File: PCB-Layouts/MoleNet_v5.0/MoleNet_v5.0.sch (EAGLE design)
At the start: 29 parts, among them Q1 MOSFET-NCHANNELBSS138, U1 STM32L073RZT6, U2 SN74LVC1G240DBVR, X1 734120110, Y1 16MHz

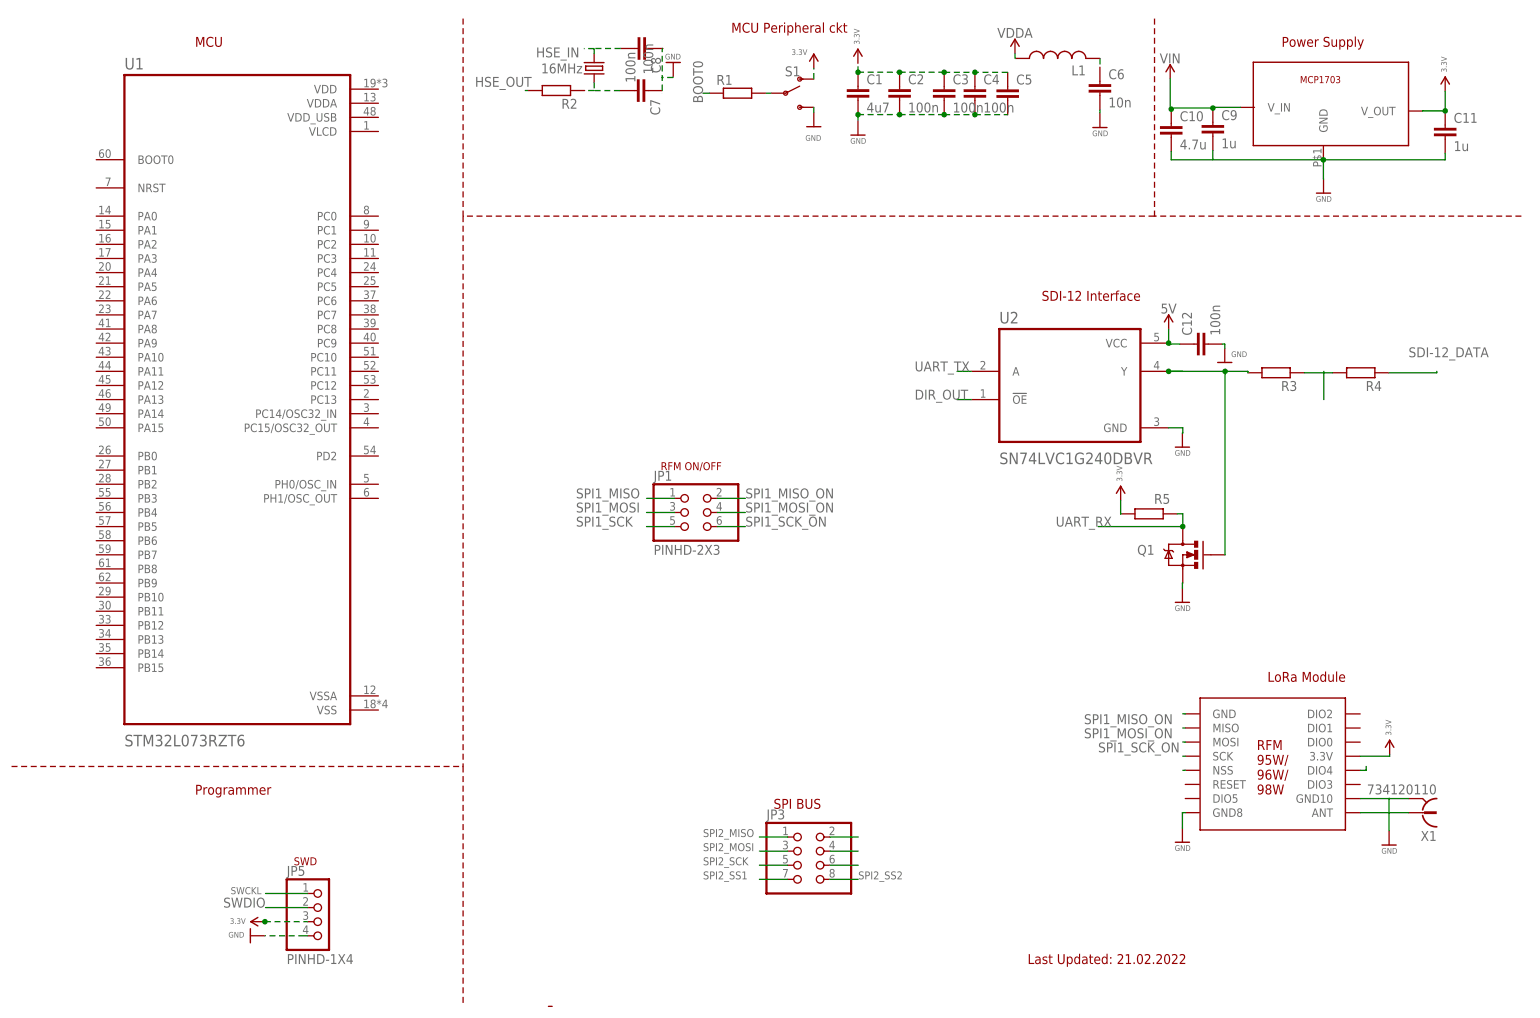
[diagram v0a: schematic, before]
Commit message: MoleNet_v5 PCB Schematic updated
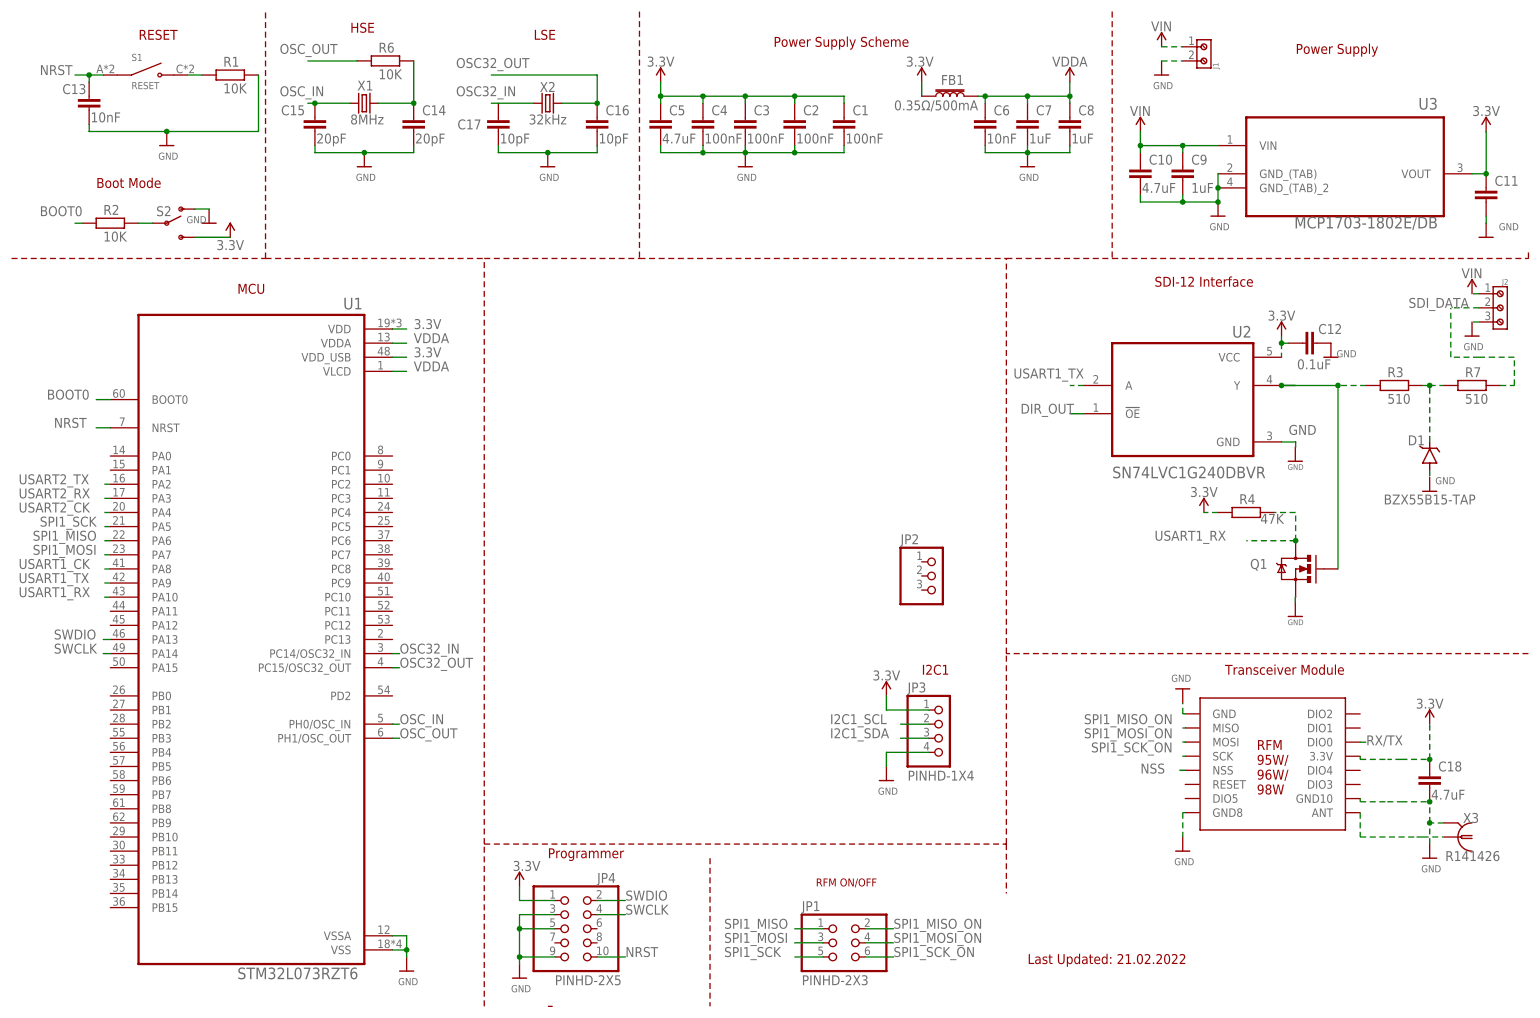
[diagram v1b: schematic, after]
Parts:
- removed JP5: PINHD-1X4, Connector:PINHD-1X4
- removed L1: (no value), rcl:L-US0204/7
- removed R5: (no value), rcl:R-EU_0204/5
- removed U$16: MCP1703_SOT23_3L, MCP1703_SOT23_3L:MCP1703_SOT23_3L
- removed Y1: 16MHz, SparkFun-Clocks:CRYSTAL-16MHZPTH-HC49US
- added C13: 10nF, rcl:C-EUC0805
- added C14, C15: 20pF, rcl:C-EUC0805
- added C16, C17: 10pF, rcl:C-EUC0805
- added C18: 4.7uF, rcl:C-EUC0805
- added D1: BZX55B15-TAP, Diodes-2:BZX55B15-TAP
- added FB1: 0.35Ω/500mA, SparkFun-Coils:FERRITE_BEAD-0603
- added J1: (no value), Wurth_Connectors_WR-TBL Rising Cage Clamp:691216710002
- added J2: (no value), Wurth_Connectors_WR-TBL Rising Cage Clamp:691216510003S
- added JP2: (no value), adafruit:PINHD-1X3
- added JP4: PINHD-2X5, Connector:PINHD-2X5
- added R6: 10K, resistor:R-EU_R0805
- added R7: 510, resistor:R-EU_R0805
- added S2: (no value), SparkFun-Retired:SWITCH-SPDTSMD
- added U3: MCP1703-1802E/DB, MCP1703-1802E_DB:MCP1703-1802E/DB
- added X2: 32kHz, SparkFun-Clocks:CRYSTAL-32.768KHZSMD-3.2X1.5
- added X3: R141426, con-coax:R141426
- C1: value 4u7 -> 100nF; device rcl:C-EU025-024X044 -> rcl:C-EUC0805
- C10: value 4.7u -> 4.7uF; device rcl:C-EU025-024X044 -> rcl:C-EUC0805
- C11: value 1u -> (none); device rcl:C-EU025-024X044 -> rcl:C-EUC0805
- C12: value 100n -> 0.1uF; device rcl:C-EU025-024X044 -> rcl:C-EUC0805
- C2, C3, C4: value 100n -> 100nF; device rcl:C-EU025-024X044 -> rcl:C-EUC0805
- C5: value (none) -> 4.7uF; device rcl:C-EU025-024X044 -> rcl:C-EUC0805
- C6: value 10n -> 10nF; device rcl:C-EU025-024X044 -> rcl:C-EUC0805
- C7, C8: value 100n -> 1uF; device rcl:C-EU025-024X044 -> rcl:C-EUC0805
- C9: value 1u -> 1uF; device rcl:C-EU025-024X044 -> rcl:C-EUC0805
- JP3: value (none) -> PINHD-1X4; device adafruit:PINHD-2X4 -> Connector:PINHD-1X4
- R1, R2: value (none) -> 10K; device rcl:R-EU_0204/5 -> resistor:R-EU_R0805
- R3: value (none) -> 510; device rcl:R-EU_0204/5 -> resistor:R-EU_R0805
- R4: value (none) -> 47K; device rcl:R-EU_0204/5 -> resistor:R-EU_R0805
- S1: value (none) -> RESET; device SparkFun-Switches:SWITCH-SPDT-PTH-11.6X4.0MM -> TS-1187A-B-A-B:TS-1187A-B-A-B
- X1: value 734120110 -> 8MHz; device con-coax:734120110 -> crystal:CRYSTALHC49S
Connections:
- net N$13 renamed NSS
- net N$17 renamed I2C1_SCL
- net SPI2_MOSI renamed I2C1_SDA
- removed net HSE_IN: Y1.1
- removed net HSE_OUT: R2.2
- removed net N$10: U$18.ANT, X1.1
- removed net N$11: U$18.GND10, X1.2
- removed net N$12: R3.1, R4.2
- removed net N$16: U$18.DIO4
- removed net N$18: JP3.4
- removed net N$19: JP3.6
- removed net N$7: C7.1, C8.1
- removed net N$8: U$18.GND
- removed net N$9: C9.2
- removed net SDI-12_DATA: R4.1
- removed net SPI2_MISO: JP3.1
- removed net SPI2_SCK: JP3.5
- removed net SPI2_SS1: JP3.7
- removed net SPI2_SS2: JP3.8
- removed net SWCKL: JP5.1
- removed net UART_RX: Q1.D, R5.1
- removed net UART_TX: U2.A
- new net NRST: C13.1, JP4.10, S1.COM, U1.NRST
- new net OSC32_IN: C17.1, U1.PC14/OSC32_IN, X2.1
- new net OSC32_OUT: C16.1, U1.PC15/OSC32_OUT, X2.2
- new net OSC_IN: C15.1, U1.PH0/OSC_IN, X1.1
- new net OSC_OUT: R6.1, U1.PH1/OSC_OUT
- new net RX/TX: U$18.DIO0
- new net SDI_DATA: J2.2, R7.2
- new net SWCLK: JP4.4, U1.PA14
- new net USART1_CK: U1.PA8
- new net USART1_RX: Q1.D, R4.2, U1.PA10
- new net USART1_TX: U1.PA9, U2.A
- new net USART2_CK: U1.PA4
- new net USART2_RX: U1.PA3
- new net USART2_TX: U1.PA2
- net 3.3V: now also C12.2, C18.1, FB1.1, JP3.1, JP4.1, R4.1, S2.S, U1.VDD, U1.VDD_USB, U2.VCC, U3.VOUT; no longer JP5.3, R5.2, S1.O, U$16.V_OUT
- net BOOT0: now also R2.1, U1.BOOT0; no longer R1.1
- net GND: now also C12.1, C13.2, C14.2, C15.2, C16.2, C17.2, C18.2, C7.2, C8.2, C9.2, D1.A, J1.2, J2.3, JP3.4, JP4.3, JP4.5, JP4.9, R1.2, S2.O, U$18.GND, U$18.GND10, U1.VSS, U1.VSSA, U3.GND_(TAB), U3.GND_(TAB)_2, X3.2; no longer C12.2, JP5.4, S1.S, U$16.GND
- net N$1: now also R1.1, S1.NO; no longer R1.2, S1.P
- net N$2: now also D1.C, R3.2, R7.1; no longer C6.1, L1.2
- net N$3: now also R3.1; no longer R3.2
- net N$4: now also R2.2, S2.P; no longer R2.1, Y1.2
- net N$5: now also C14.1, R6.2, X1.2; no longer C7.2
- net N$6: now also U$18.ANT, X3.1; no longer C8.2
- net SPI1_MISO: now also U1.PA6
- net SPI1_MOSI: now also U1.PA7
- net SPI1_SCK: now also U1.PA5
- net SWDIO: now also JP4.2, U1.PA13; no longer JP5.2
- net VDDA: now also C6.1, C7.1, C8.1, FB1.2, U1.VDDA, U1.VLCD; no longer L1.1
- net VIN: now also J1.1, J2.1, U3.VIN; no longer C12.1, U$16.V_IN, U2.VCC
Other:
- note added: "Boot Mode"
- note added: "HSE"
- note added: "I2C1"
- note added: "LSE"
- note added: "Power Supply Scheme"
- note added: "RESET"
- note added: "Transceiver Module"
- note removed: "LoRa Module"
- note removed: "MCU Peripheral ckt"
- note removed: "SPI BUS"
- note removed: "SWD"
- moved on the sheet: C1, C10, C11, C12, C2, C3, C4, C5, C6, C7, C8, C9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
